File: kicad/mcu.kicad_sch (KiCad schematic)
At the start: 9 parts

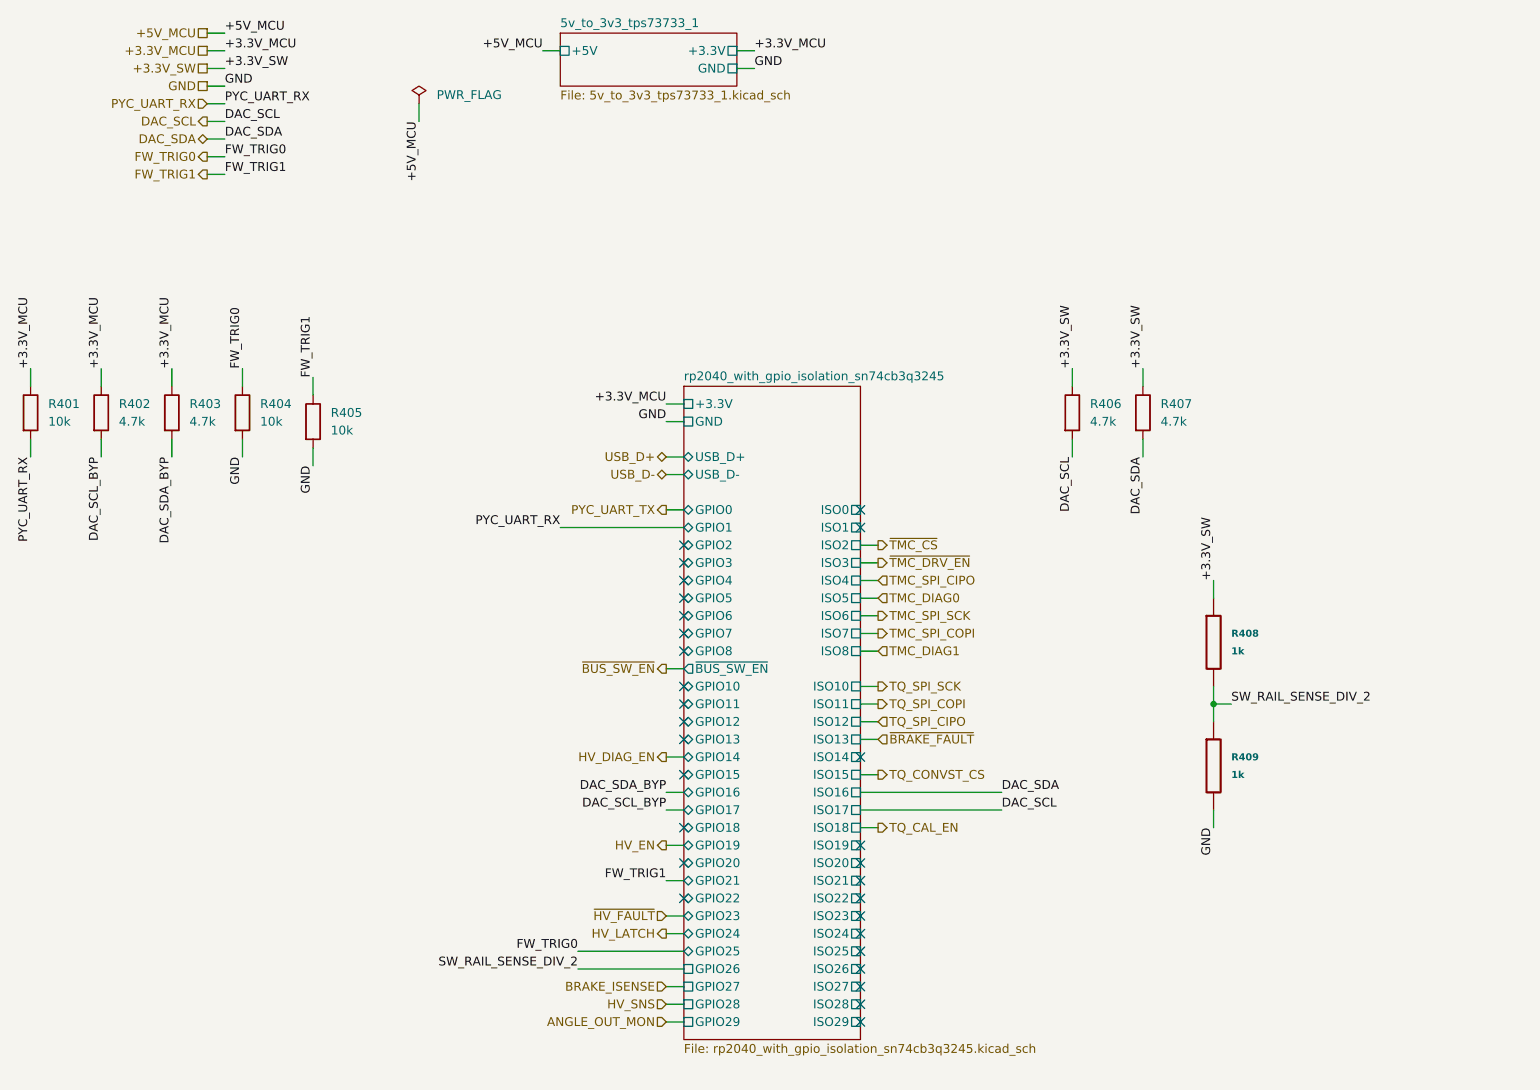
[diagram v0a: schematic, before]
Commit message: Add inst resistor to rp2040 block
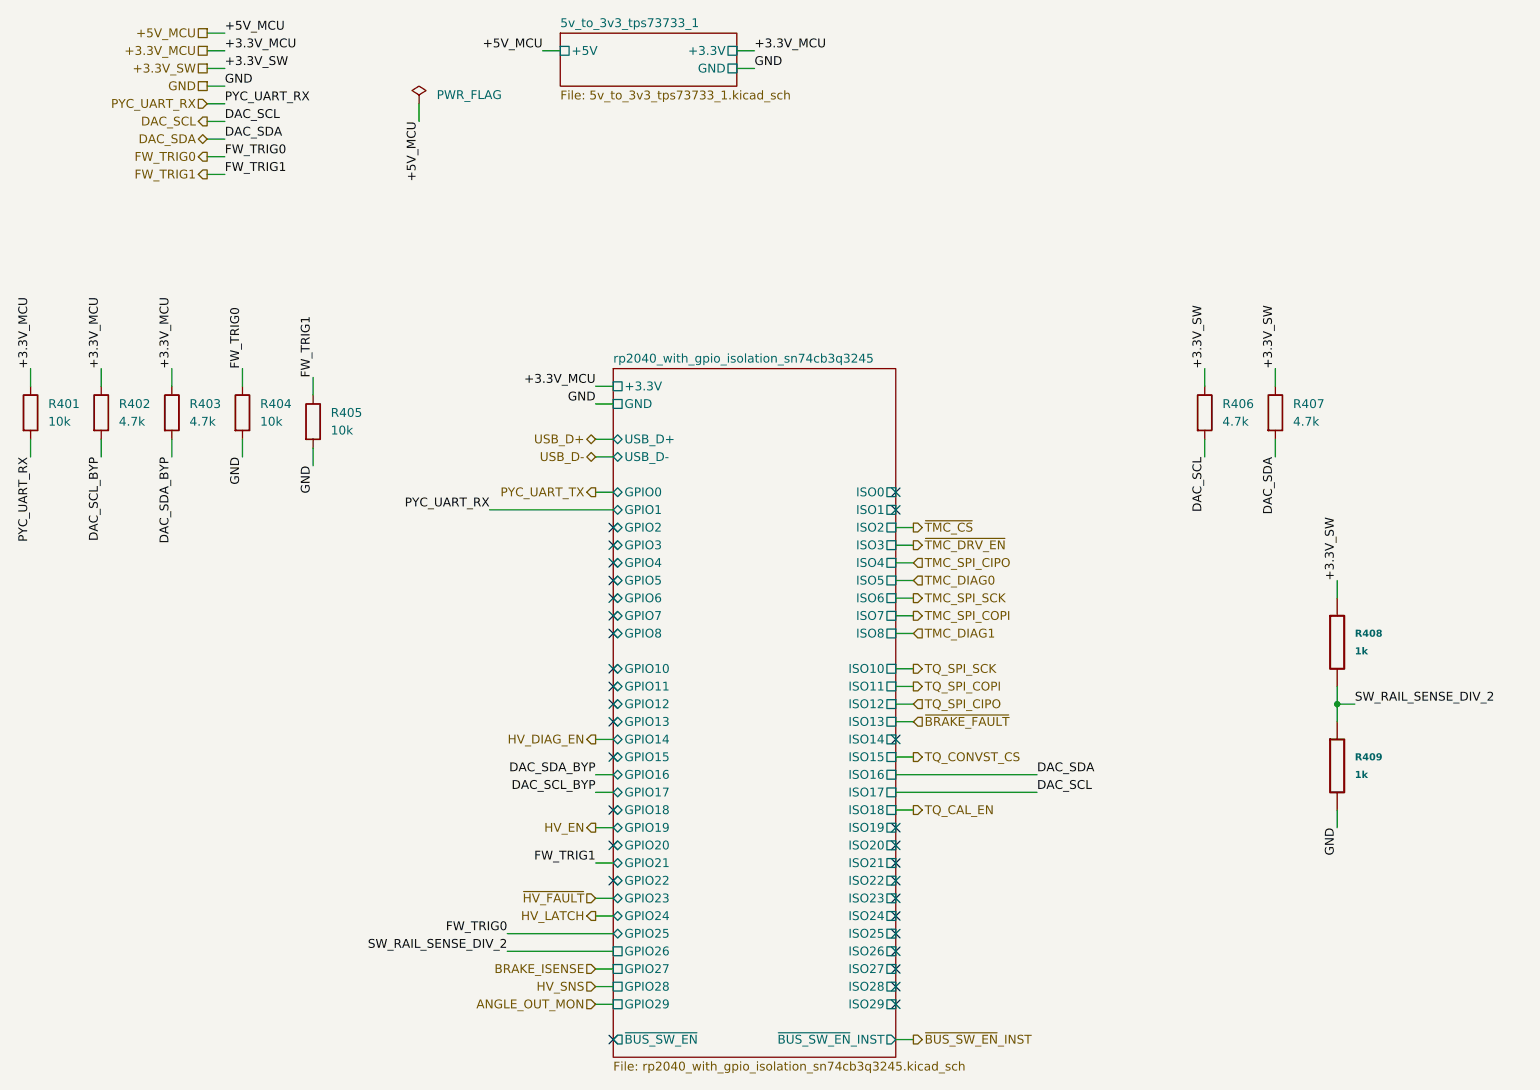
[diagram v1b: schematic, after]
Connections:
- no-connect marks 29 -> 30
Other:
- sheet rp2040_with_gpio_isolation_sn74cb3q3245 ports: added ~{BUS_SW_EN}_INST; removed none
- moved on the sheet: R406, R407, R408, R409
